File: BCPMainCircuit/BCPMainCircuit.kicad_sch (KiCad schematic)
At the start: 14 parts, among them Q1 PMOS, SW1 SW_Nidec_CAS-120A1, U1 LD1117V33, U2 Pico 2, U3 DEV-13712, U6 BME280

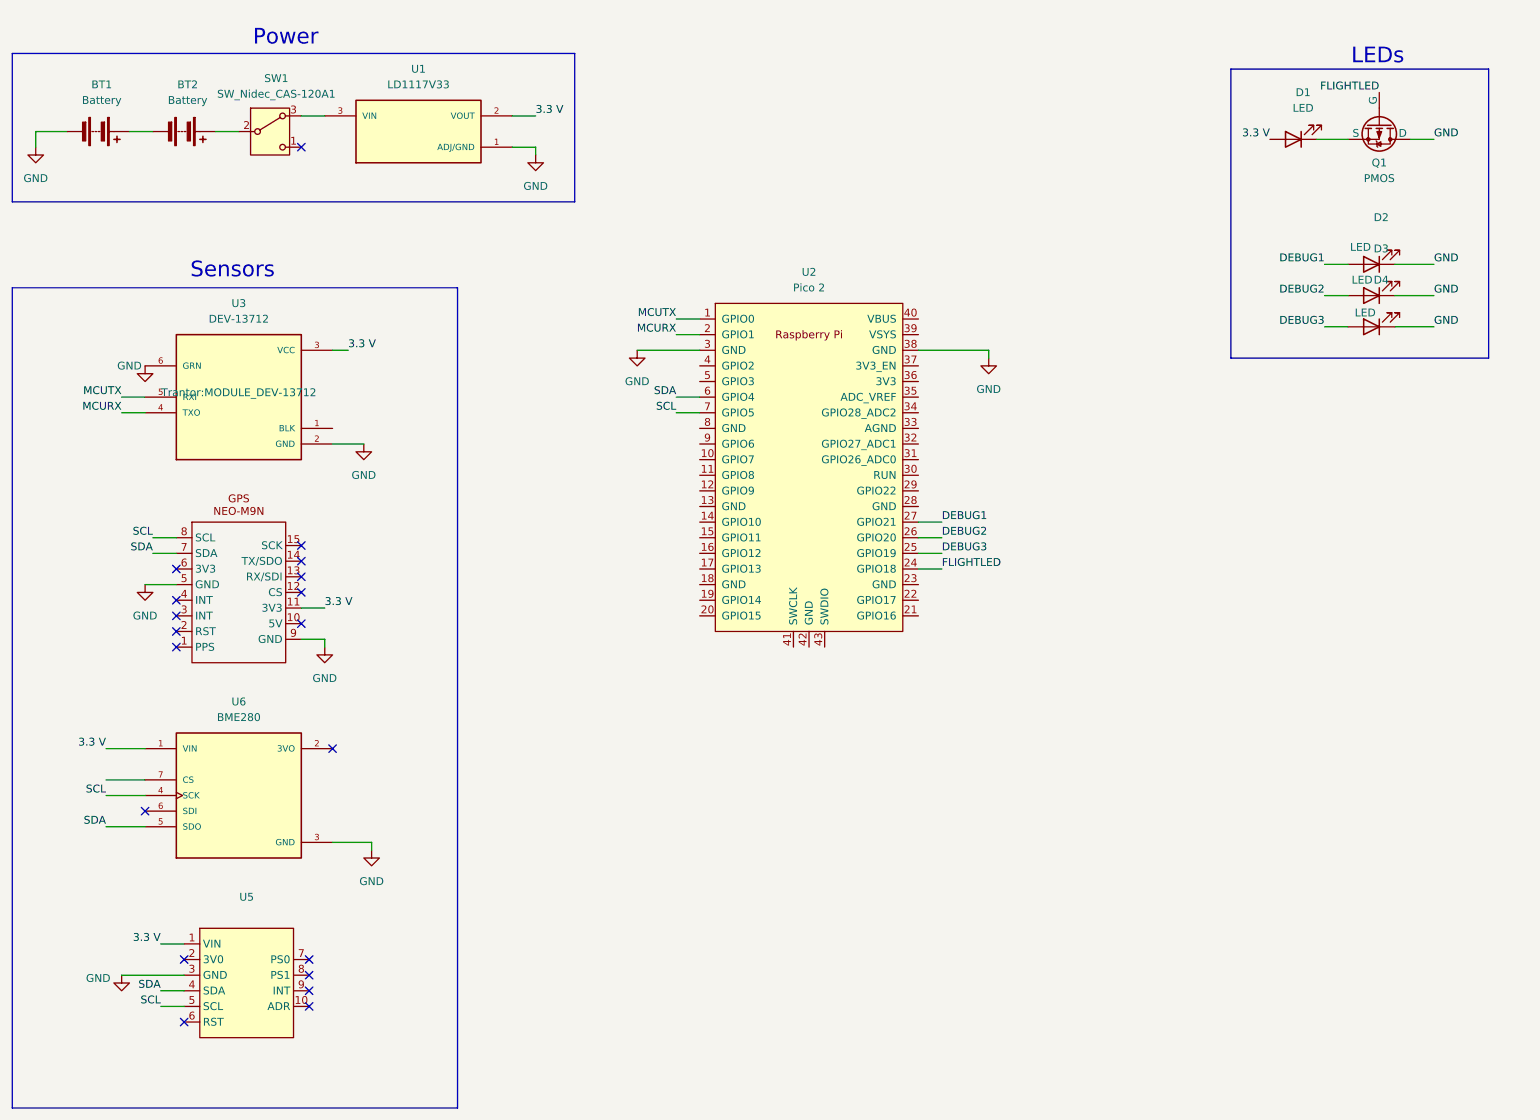
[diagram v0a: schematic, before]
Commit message: Minor Changes
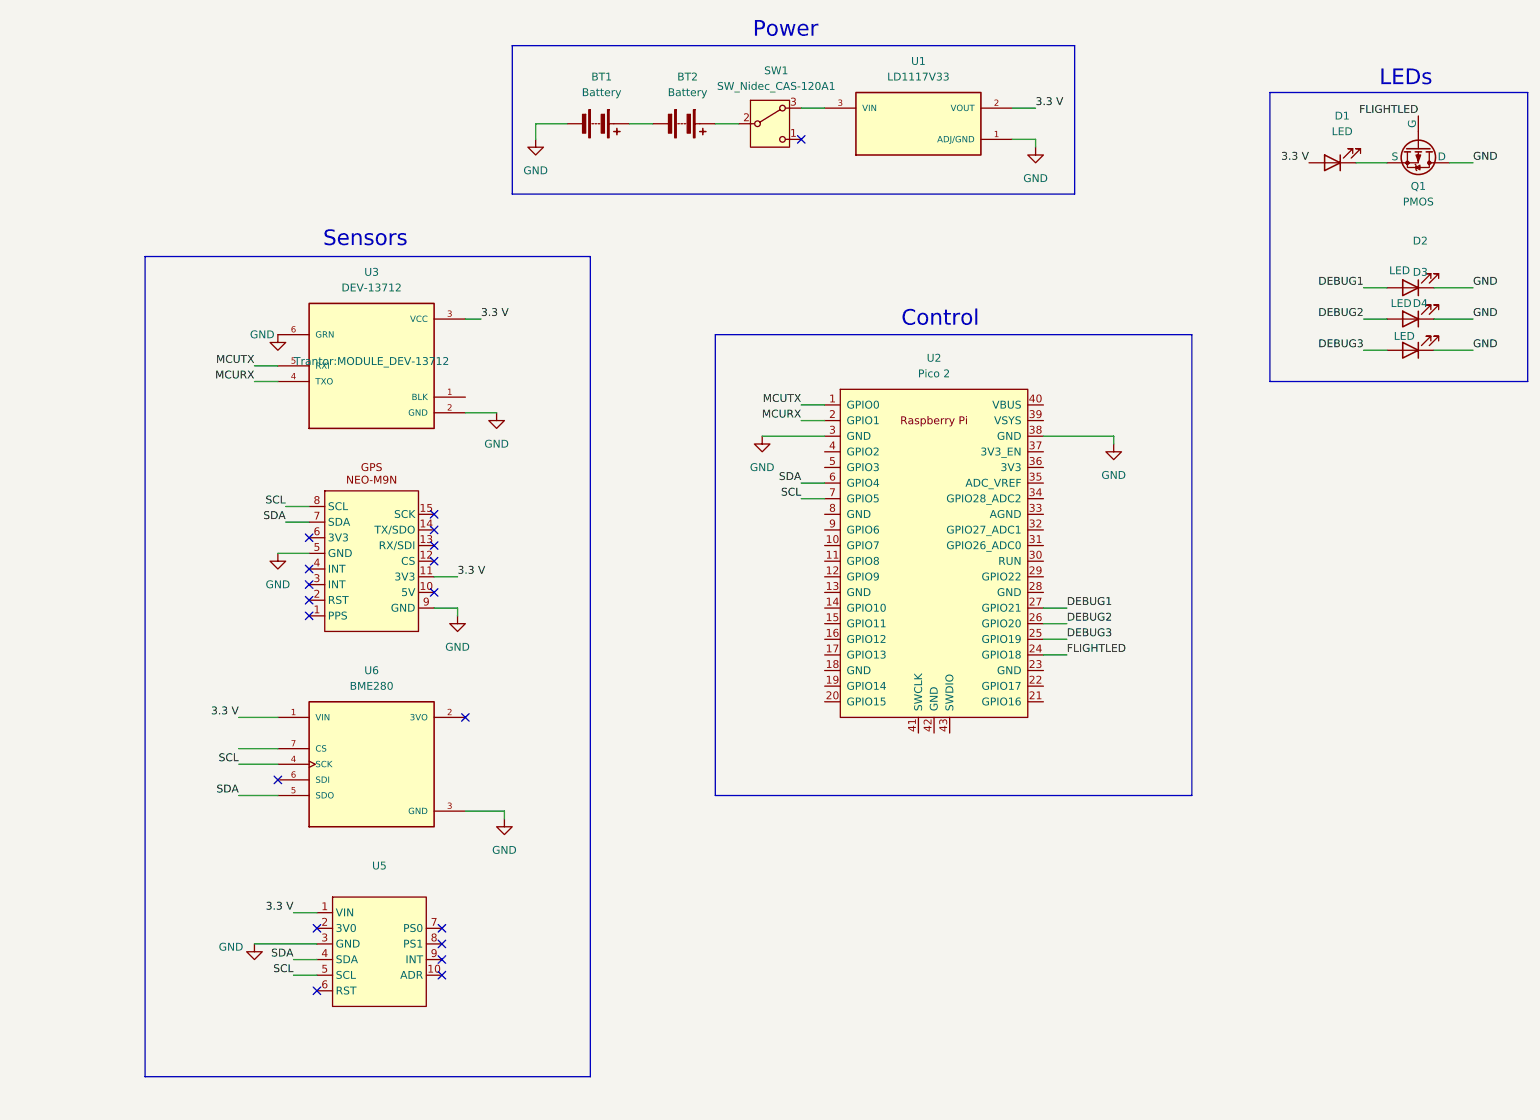
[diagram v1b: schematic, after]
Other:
- note added: "Control"
- company: (none) -> TRANTOR Orbital Research Group
- title: (none) -> BCP Main Circuit
- moved on the sheet: BT1, BT2, D1, D2, D3, D4, Q1, SW1, U1, U2, U3, U5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
